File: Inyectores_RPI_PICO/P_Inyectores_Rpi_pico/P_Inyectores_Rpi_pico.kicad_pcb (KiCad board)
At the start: 2 copper layers, 100 x 100 mm, 87 parts, among them J1 Entrada_12V/4A, K1 SANYOU_SRD_Form_C, K2 SANYOU_SRD_Form_C, Q1 IRF540N, Q2 IRF540N, Q3 IRF540N, Q4 IRF540N, Q5 BC548, Q6 BC548, Q7 BC548, SW2 Reset_Push, SW3 Rotary_Encoder_Switch, U1 PC817, U10 DS3231M, U11 AT24CS32-XHM, U2 PC817, U3 PC817, U4 PC817, U5 L7805, U6 AMS1117-3.3, U7 Pico, U8 PC817, U9 PC817

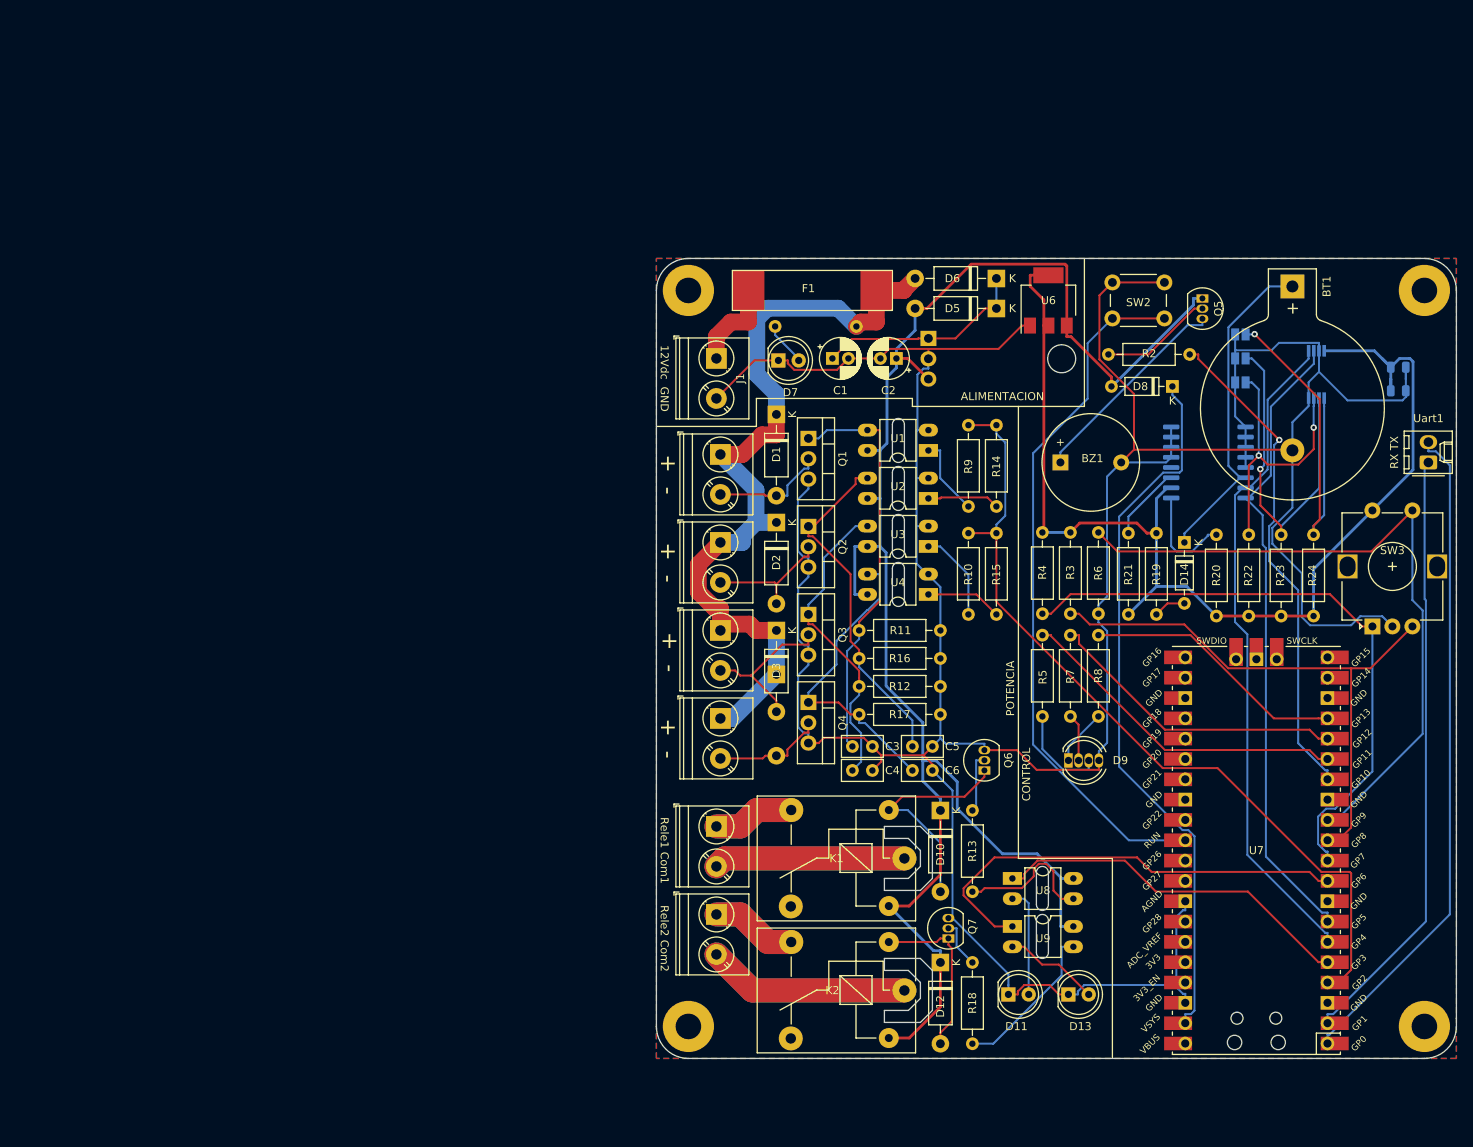
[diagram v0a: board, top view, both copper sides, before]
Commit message: Actualizacion PCB
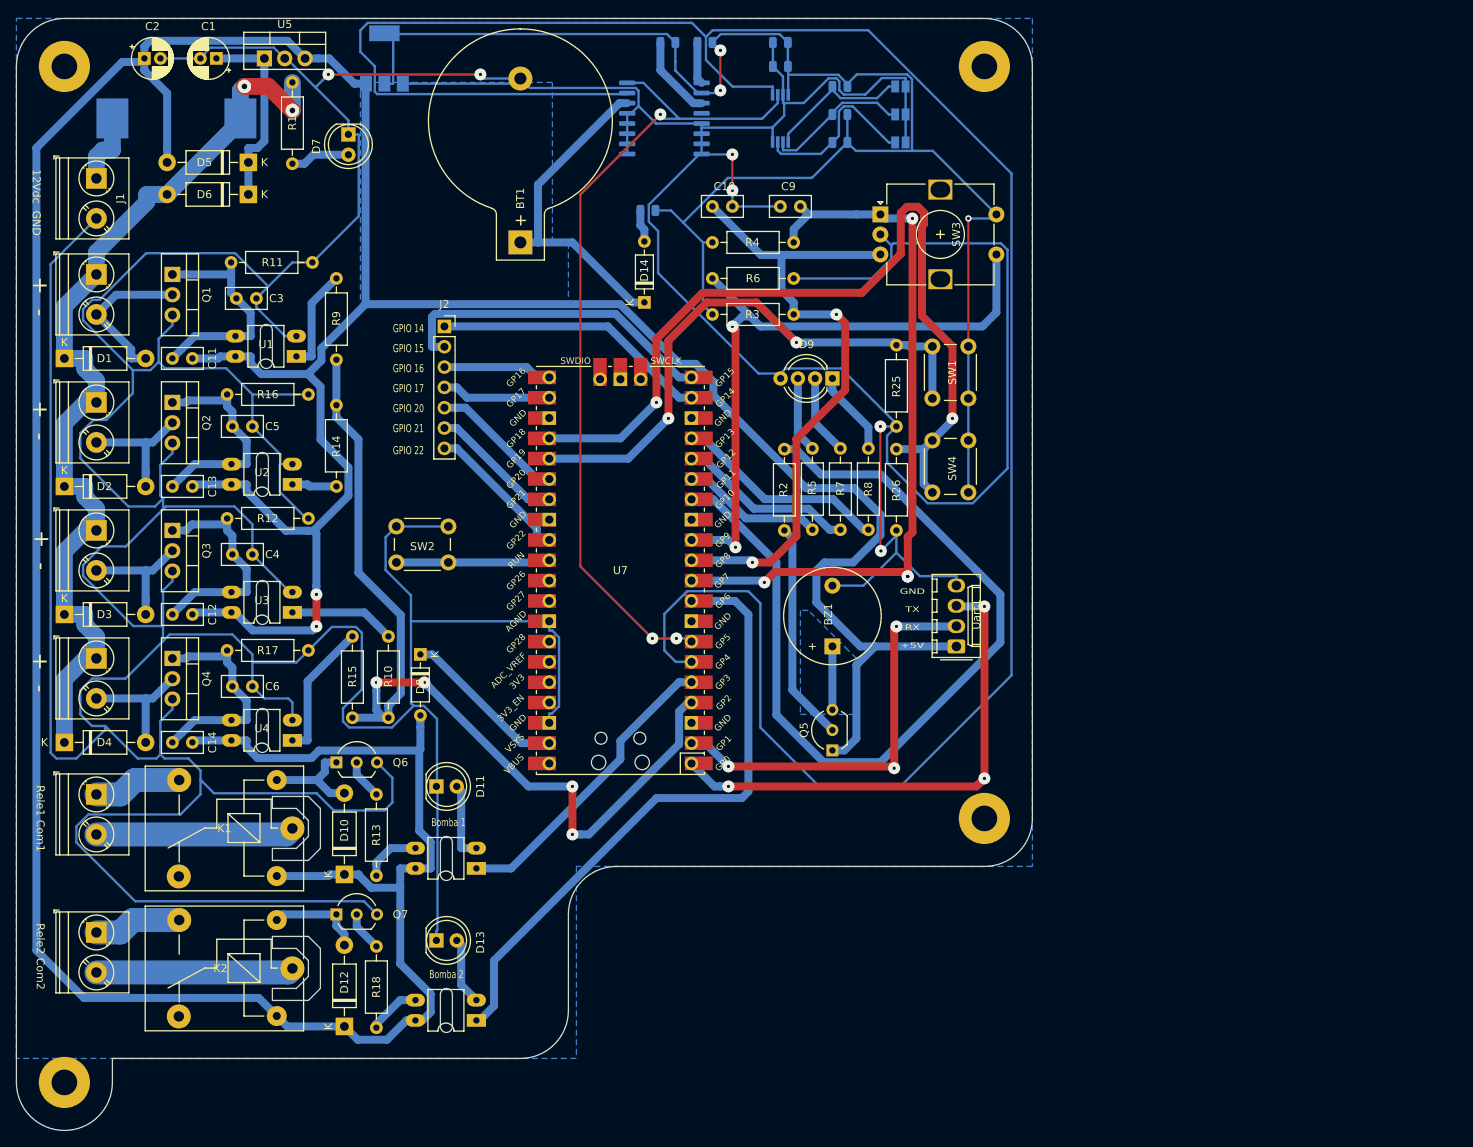
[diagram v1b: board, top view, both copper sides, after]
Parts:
- added C10: 104, Capacitor_THT:C_Disc_D5.0mm_W2.5mm_P2.50mm, F.Cu at (107.0, 43.5)
- added C11: 104, Capacitor_THT:C_Disc_D5.0mm_W2.5mm_P2.50mm, F.Cu at (42.0, 62.5)
- added C12: 104, Capacitor_THT:C_Disc_D5.0mm_W2.5mm_P2.50mm, F.Cu at (42.0, 94.5)
- added C13: 104, Capacitor_THT:C_Disc_D5.0mm_W2.5mm_P2.50mm, F.Cu at (42.0, 78.5)
- added C14: 104, Capacitor_THT:C_Disc_D5.0mm_W2.5mm_P2.50mm, F.Cu at (42.0, 110.5)
- added C9: 104, Capacitor_THT:C_Disc_D5.0mm_W2.5mm_P2.50mm, F.Cu at (118.0, 43.5)
- added J2: Conn_01x07_Male, Connector_PinSocket_2.54mm:PinSocket_1x07_P2.54mm_Vertical, F.Cu at (73.5, 58.5)
- added R25: 10k, Resistor_THT:R_Axial_DIN0207_L6.3mm_D2.5mm_P10.16mm_Horizontal, F.Cu at (130.0, 71.0)
- added R26: 10k, Resistor_THT:R_Axial_DIN0207_L6.3mm_D2.5mm_P10.16mm_Horizontal, F.Cu at (130.0, 84.0)
- added SW1: PUSH2, Button_Switch_THT:SW_PUSH_6mm, F.Cu at (139.0, 61.0)
- added SW4: PUSH1, Button_Switch_THT:SW_PUSH_6mm, F.Cu at (139.0, 72.8)
- D4, R1: moved to F.Cu
- D9: footprint LED_THT:LED_D5.0mm-4_RGB -> LED_THT:LED_D5.0mm-4_RGB_Wide_Pins
- F1, U6: moved to B.Cu
- Q5, Q6, Q7: footprint Package_TO_SOT_THT:TO-92_Inline -> Package_TO_SOT_THT:TO-92_Inline_Wide
- R13: value R -> 12k
- R19, R20, R21, R22, R23, R24: footprint Resistor_THT:R_Axial_DIN0207_L6.3mm_D2.5mm_P10.16mm_Horizontal -> Resistor_SMD:R_0805_2012Metric; moved to B.Cu
- R2: value 53k -> 4k7
- U5: footprint Package_TO_SOT_THT:TO-220-3_Horizontal_TabUp -> Package_TO_SOT_THT:TO-220-3_Vertical; moved to F.Cu
- Uart1: footprint Connector_Molex:Molex_KK-254_AE-6410-02A_1x02_P2.54mm_Vertical -> Connector_Molex:Molex_KK-254_AE-6410-04A_1x04_P2.54mm_Vertical
- moved Tornillo4 132.0 mm to (141.0, 26.0)
- moved C2 101.2 mm to (36.0, 25.0), turned to 0 degrees
- moved D8 99.8 mm to (70.5, 99.5), turned to 270 degrees
- moved BT1 96.7 mm to (83.0, 48.0), turned to 90 degrees
- moved R20 96.1 mm to (106.1, 23.0), turned to 180 degrees
- moved D5 95.3 mm to (49.0, 38.0)
- moved C3 95.2 mm to (47.5, 55.0)
- moved SW2 94.6 mm to (74.0, 88.0)
- moved D6 94.1 mm to (49.0, 42.0)
- moved C5 93.9 mm to (47.0, 71.0)
- moved R21 91.8 mm to (101.4, 23.0), turned to 180 degrees
- moved R11 91.0 mm to (57.0, 50.5)
- moved U5 90.1 mm to (51.0, 25.0), turned to 0 degrees
- moved D4 89.4 mm to (26.0, 110.5), turned to 0 degrees
- moved D1 89.3 mm to (26.0, 62.5), turned to 0 degrees
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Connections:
- U7 pad 19: Net-(U7-Pad19) -> /Control/GPIO14
- U7 pad 20: Net-(U7-Pad20) -> /Control/GPIO15
- U7 pad 21: Net-(U7-Pad21) -> /Control/GPIO16
- U7 pad 22: Net-(U7-Pad22) -> /Control/GPIO17
- U7 pad 24: Net-(U7-Pad24) -> /Control/PULSADOR_1
- U7 pad 25: Net-(U7-Pad25) -> /Control/PULSADOR_2
- U7 pad 26: Net-(U7-Pad26) -> /Control/GPIO20
- U7 pad 27: Net-(U7-Pad27) -> /Control/GPIO21
- U7 pad 29: Net-(U7-Pad29) -> /Control/GPIO22
- Uart1 pad 1: /Control/UART0_RX -> +5V
- Uart1 pad 2: /Control/UART0_TX -> /Control/UART0_RX
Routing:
- net GND: track 450.8 -> 949.9 mm, vias 0 -> 6
- net +5V: track 216.5 -> 563.6 mm, vias 0 -> 2
- net /Control/I2C0_SDA: track 83.1 -> 284.8 mm
- net /Control/PULSADOR_1: track 0.00 -> 108.8 mm, vias 0 -> 2
- net /Control/PULSADOR_2: track 0.00 -> 70.5 mm, vias 0 -> 2
- net Net-(D8-Pad1): track 89.8 -> 20.7 mm
- net /Control/RESET: track 87.9 -> 19.2 mm
- net +3V3: track 145.9 -> 210.6 mm, vias 0 -> 3
- net /Control/Buzzer: track 62.1 -> 110.2 mm, vias 1 -> 0
- net /Control/GPIO15: track 0.00 -> 41.2 mm
- net /Control/GPIO14: track 0.00 -> 34.6 mm
- net Net-(JP1-Pad2): track 47.6 -> 18.1 mm, vias 1 -> 0
- net /Control/Com_Rele2: track 50.7 -> 24.7 mm
- net Net-(JP2-Pad2): track 43.8 -> 18.3 mm, vias 1 -> 0
- net /Control/Rgb1: track 42.1 -> 17.7 mm
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- added copper zone on B.Cu, net +5V
- added copper zone on B.Cu, net Net-(BZ1-Pad1)
- removed copper zone on F.Cu, net GND
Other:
- board size 100 x 100 mm -> 127 x 139 mm
- net class 1A: trace_width 0.35 -> 1; via_dia 0.8 -> 1.5
- net class CNC added: clearance 0.2, trace_width 1, via_dia 1.5, via_drill 0.4
- net class Control: trace_width 0.25 -> 0.3; via_dia 0.8 -> 1.5
- net class Default: via_dia 0.8 -> 1.5
- net class Rele: via_dia 0.8 -> 1.5
- board text added: "Bomba 1"
- board text added: "Bomba 2"
- board text added: "GND TX RX +5V"
- board text added: "GPIO 14"
- board text added: "GPIO 15"
- board text added: "GPIO 16"
- board text added: "GPIO 17"
- board text added: "GPIO 20"
- board text added: "GPIO 21"
- board text added: "GPIO 22"
- board text added: "Zuliani, Agustin"
- board text removed: "ALIMENTACION"
- board text removed: "CONTROL"
- board text removed: "POTENCIA"
- board text removed: "RX TX"
